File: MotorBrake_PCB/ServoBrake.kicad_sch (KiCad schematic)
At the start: 20 parts, among them CN1 XT30(2+2)PB-M.G.B, CN3 EMER, Q1 AO3400A, U1 74LVC1G08, U2 INA240A2D, U3 TPS3430WDRC

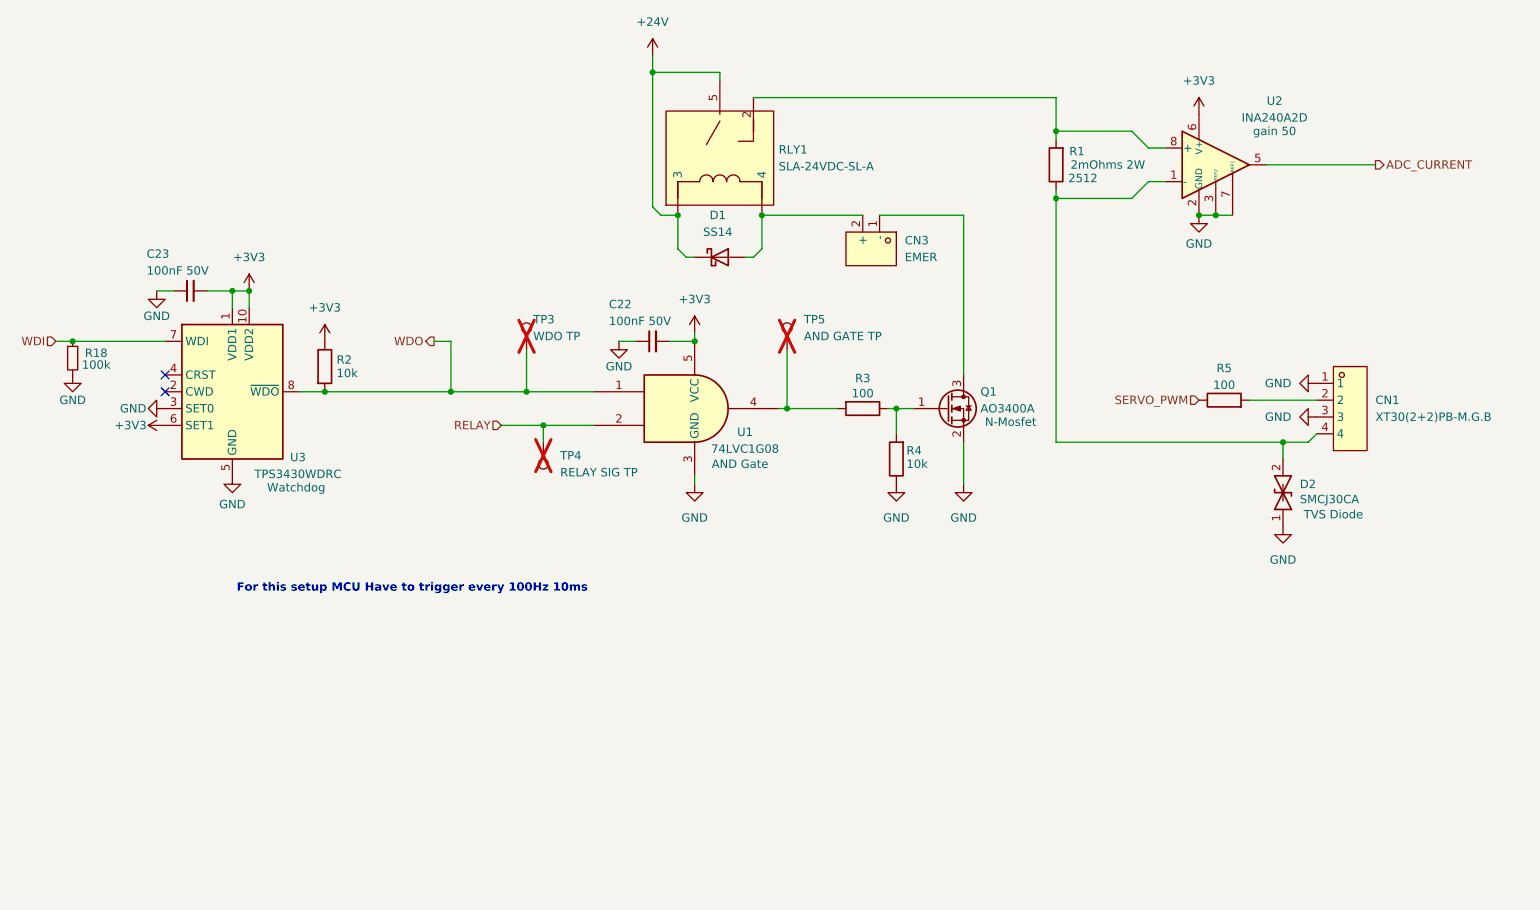
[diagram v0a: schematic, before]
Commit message: up
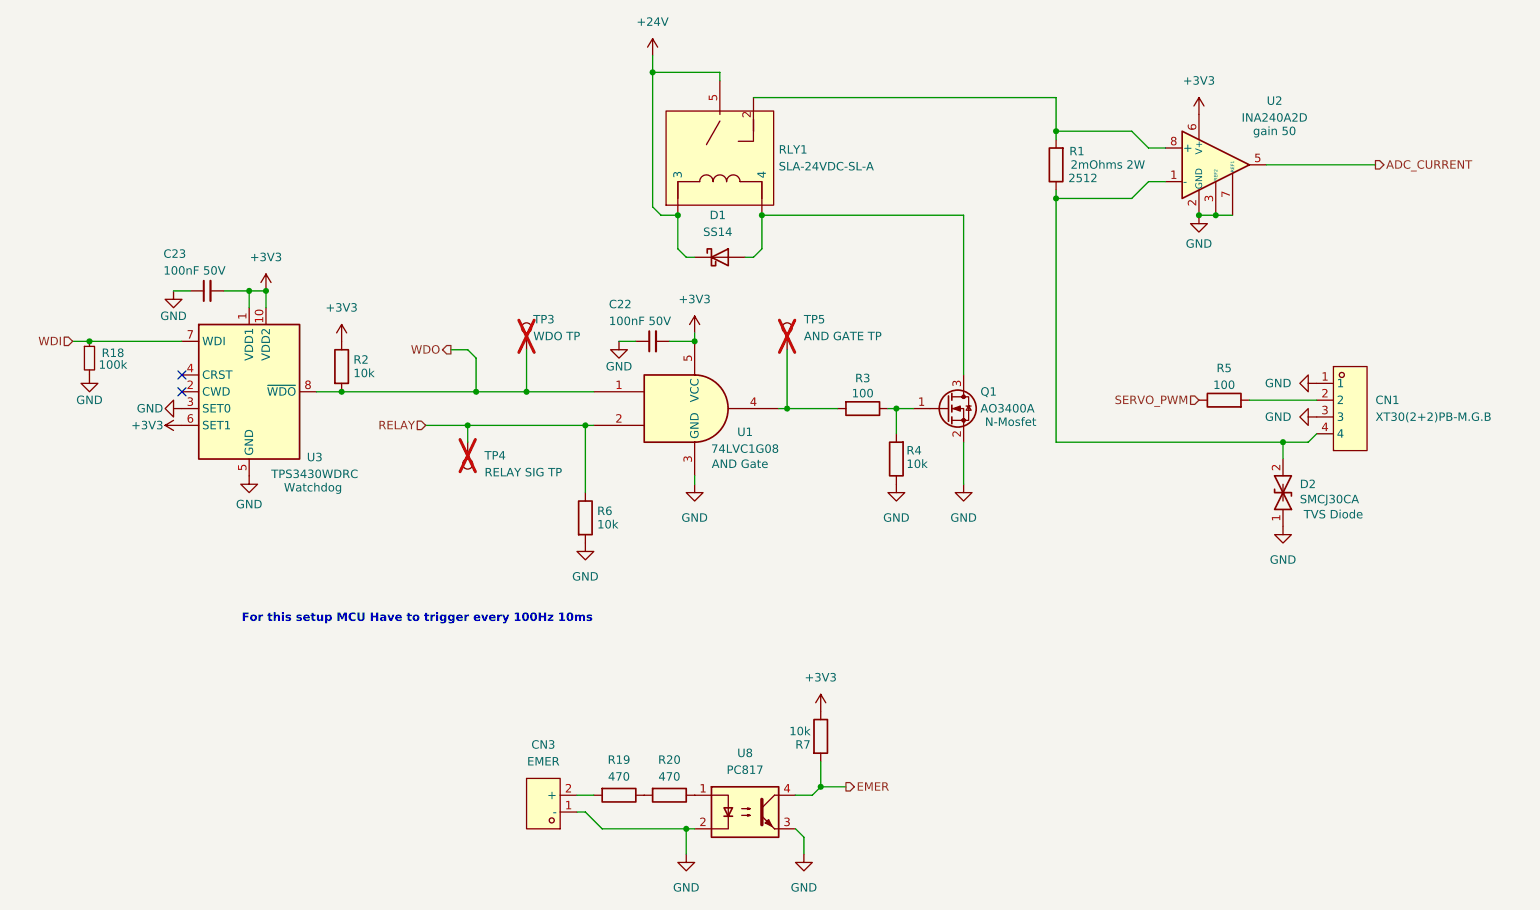
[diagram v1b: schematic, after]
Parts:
- added R19, R20: 470, Resistor_SMD:R_0603_1608Metric, symbol Device:R
- added R6, R7: 10k, Resistor_SMD:R_0402_1005Metric, symbol Device:R
- added U8: PC817, Package_DIP:DIP-4_W7.62mm, symbol Isolator:PC817
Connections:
- net +3V3: now also R7.1
- net GND: now also CN3.1 (-), R6.2, U8.2, U8.3
- net RELAY: now also R6.1
- net at D1.2 (A), RLY1.4: now also Q1.3 (D); no longer CN3.2 (+)
- new net: R19.1, R20.2
- new net: CN3.2 (+), R19.2
- new net: R20.1, U8.1
- new net EMER: R7.2, U8.4
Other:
- moved on the sheet: C23, R18, R2, TP4, U3

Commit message: Isolate B-
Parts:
- U8: FT Rotation Offset (none) -> 270
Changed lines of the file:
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@@
+			)
+		)
+		(property "FT Rotation Offset" "270"
+			(at 130.81 176.53 0)
+			(hide yes)
+			(show_name no)
+			(do_not_autoplace no)
+			(effects
+				(font
+					(size 1.27 1.27)
+				)
 			)
 		)
